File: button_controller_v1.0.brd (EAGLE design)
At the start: 160 x 100 mm, 88 parts, among them IC2 4051D, IC3 4520D, IC5 4051D

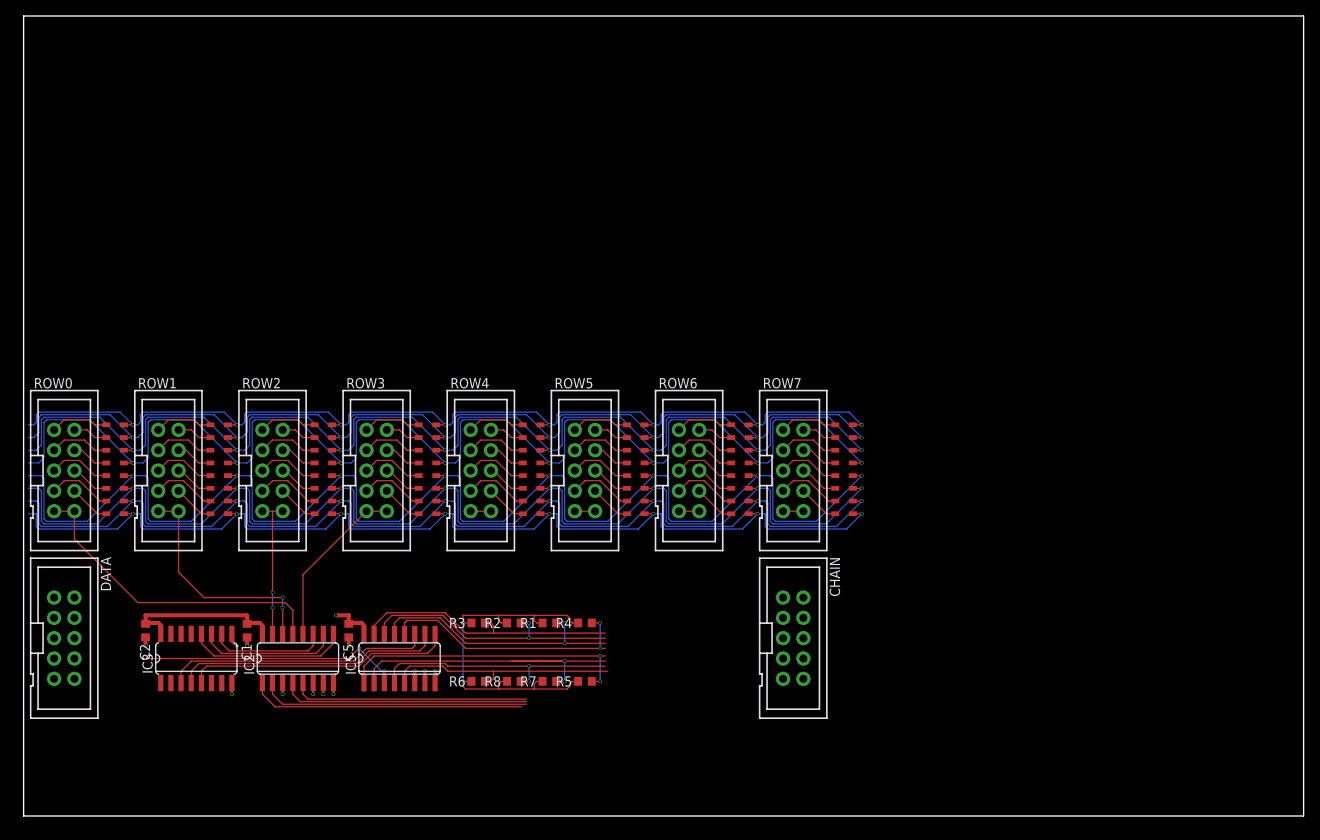
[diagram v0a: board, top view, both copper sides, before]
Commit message: Finished tracing
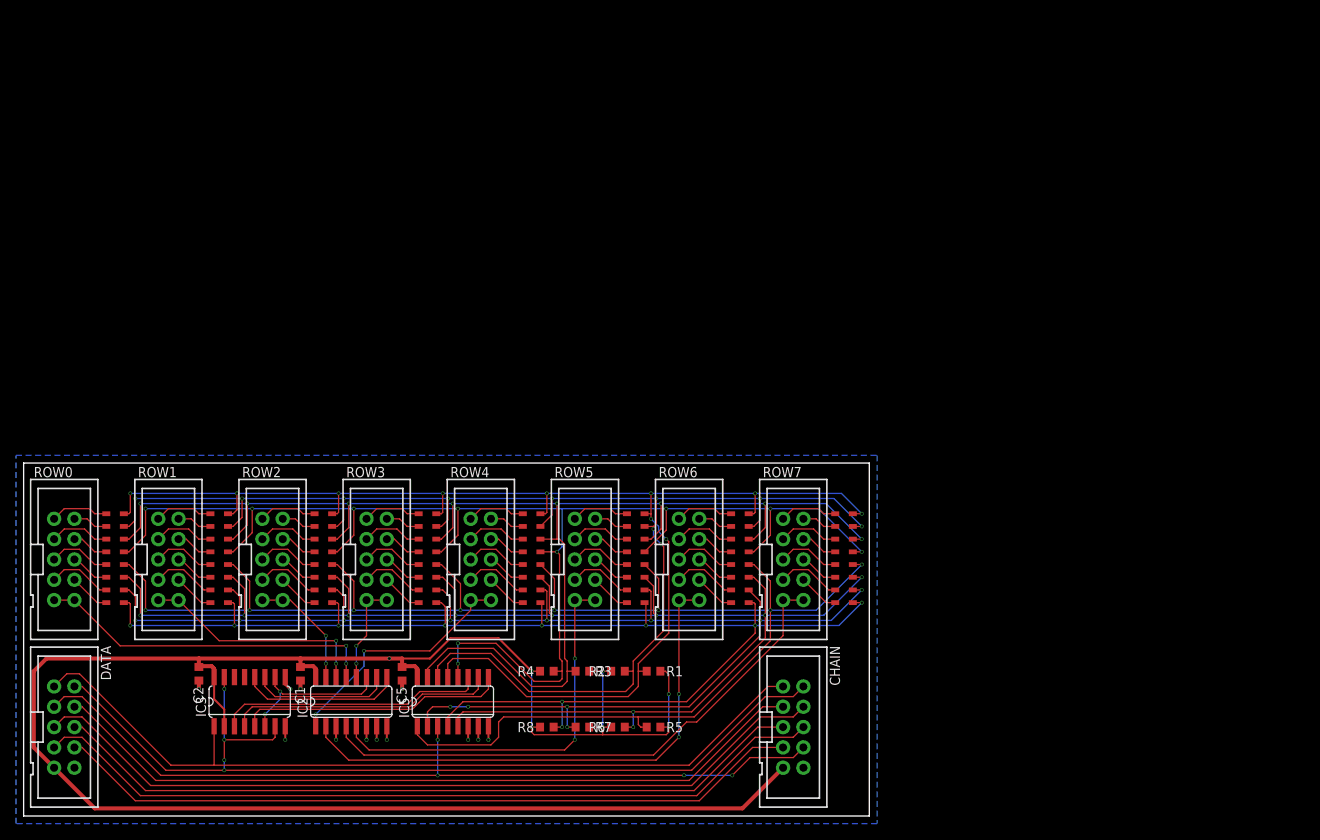
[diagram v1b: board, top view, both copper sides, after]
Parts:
- moved R6 18.4 mm to (74.3, 11.1)
- moved R1 14.3 mm to (78.7, 18.1), turned to 0 degrees
- moved R2 14.3 mm to (74.3, 18.1)
- moved R3 14.3 mm to (69.8, 18.1), turned to 0 degrees
- moved D14 11.1 mm to (11.4, 29.8)
- moved D17 11.1 mm to (37.5, 37.8)
- moved D22 11.1 mm to (37.5, 29.8)
- moved D25 11.1 mm to (24.4, 37.8)
- moved D30 11.1 mm to (24.4, 29.8)
- moved D33 11.1 mm to (63.5, 37.8)
- moved D38 11.1 mm to (63.5, 29.8)
- moved D41 11.1 mm to (50.5, 37.8)
- moved D46 11.1 mm to (50.5, 29.8)
- moved D57 11.1 mm to (76.5, 37.8)
- moved D62 11.1 mm to (76.5, 29.8)
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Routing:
- net +5V: track 75.1 -> 243.3 mm, vias 3 -> 7
- net RESET: track 0.00 -> 119.3 mm, vias 0 -> 4
- net CLK: track 0.00 -> 105.5 mm
- net BUTTON_VAL_CHAIN_2: track 0.00 -> 101.8 mm
- net BUTTON_VAL_CHAIN_4: track 0.00 -> 100.8 mm
- net BUTTON_VAL_CHAIN_1: track 0.00 -> 96.2 mm
- net BUTTON_VAL_CHAIN_3: track 0.00 -> 95.2 mm
- net BUTTON_VAL_CHAIN_5: track 0.00 -> 94.1 mm
- net BUTTON_VALUE: track 32.7 -> 105.8 mm, vias 2 -> 4
- net ROW7: track 33.5 -> 70.1 mm
- net ROW6: track 36.2 -> 67.6 mm, vias 0 -> 2
- net COL3: track 202.0 -> 178.3 mm
- net ROW5: track 32.1 -> 49.9 mm, vias 0 -> 2
- net COL2: track 189.1 -> 176.0 mm
- net COL4: track 212.9 -> 200.3 mm, vias 10 -> 8
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- added copper zone on layer 16, net GND
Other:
- board size 160 x 100 mm -> 105.7 x 44.1 mm
